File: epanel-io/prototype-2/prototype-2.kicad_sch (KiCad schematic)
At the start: 30 parts, among them J1 Conn_01x05_Male, J2 Screw_Terminal_01x04, J3 Screw_Terminal_01x04, J4 Screw_Terminal_01x02, Q1 IRF830, Q2 IRF830, SW1 SW_Push, U1 Pico, U2 4N35, U3 4N35, U4 H11AA1, U5 H11AA1, U6 H11AA1

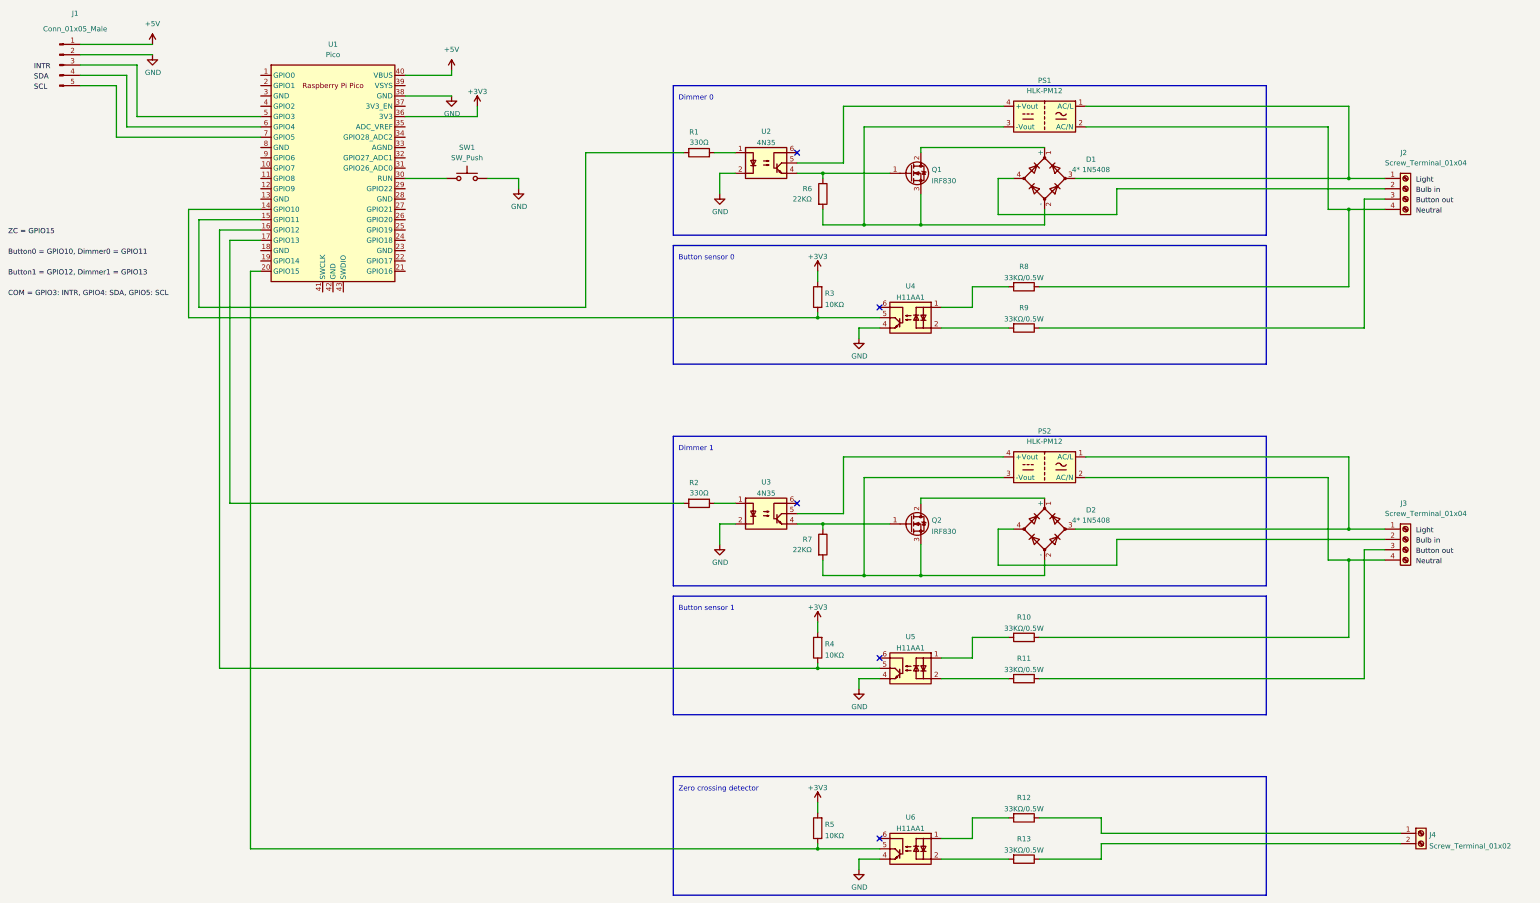
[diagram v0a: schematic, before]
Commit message: remove pico from pcb
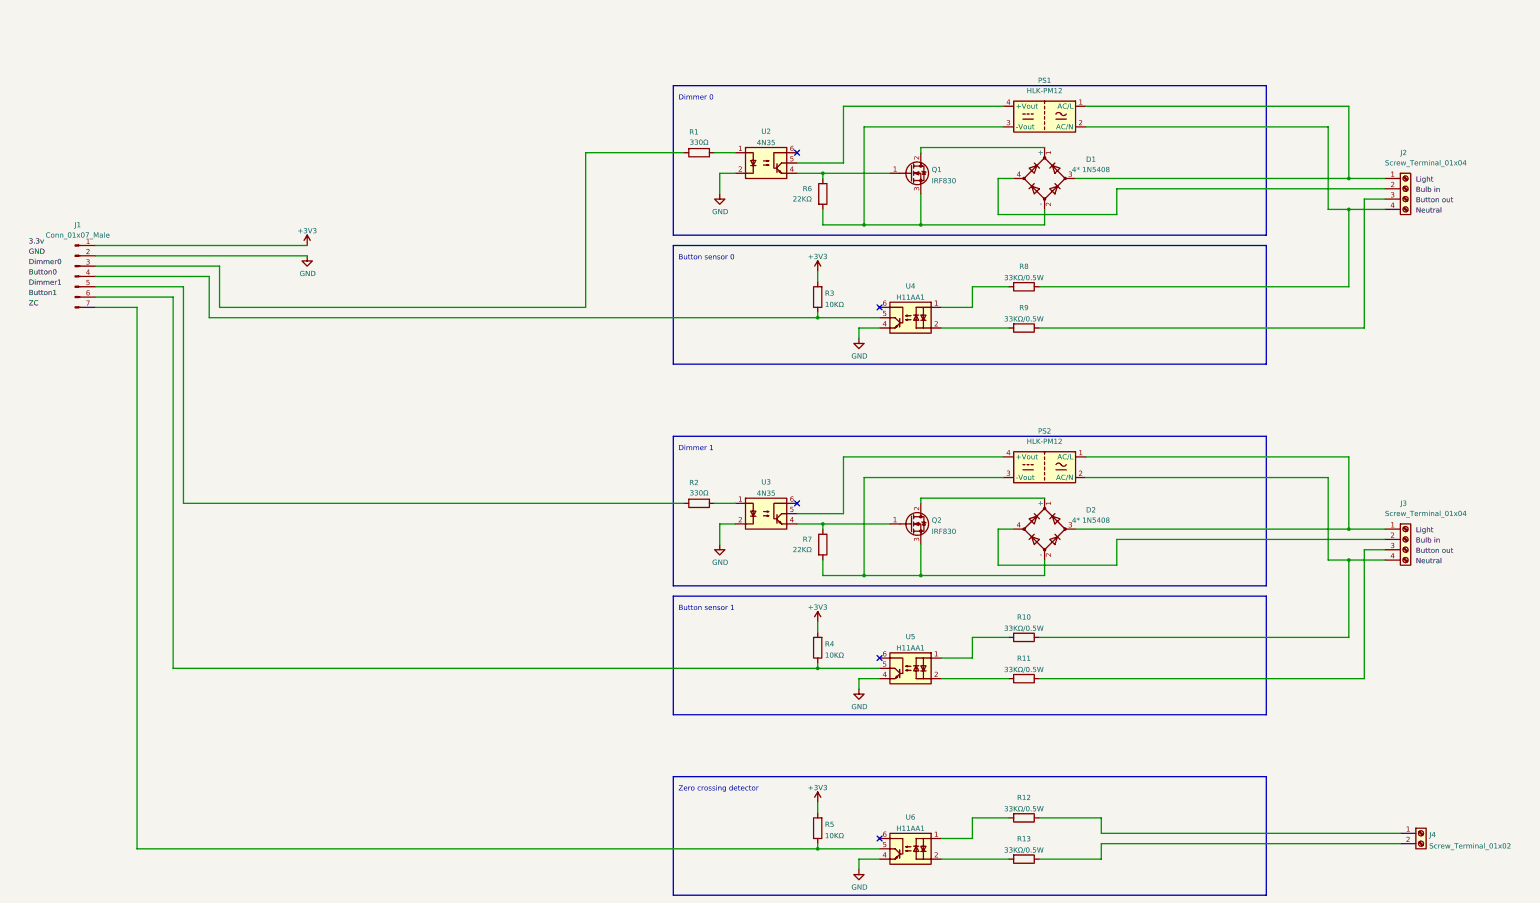
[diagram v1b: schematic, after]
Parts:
- removed J1: Conn_01x05_Male, Connector_PinHeader_2.54mm:PinHeader_1x05_P2.54mm_Vertical, symbol Connector:Conn_01x05_Male
- removed SW1: SW_Push, Button_Switch_SMD:SW_SPST_REED_CT05-XXXX-J1, symbol Switch:SW_Push
- removed U1: Pico, MCU_RaspberryPi_and_Boards:RPi_Pico_SMD_TH, symbol MCU_RaspberryPi_and_Boards:Pico
- added J1: Conn_01x07_Male, symbol Connector:Conn_01x07_Male
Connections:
- net +3V3: now also J1.1 (Pin_1)
- net GND: now also J1.2 (Pin_2)
- net at R4.1, U5.5: now also J1.6 (Pin_6)
- net at R1.2: now also J1.3 (Pin_3)
- net at R3.1, U4.5: now also J1.4 (Pin_4)
- net at R2.2: now also J1.5 (Pin_5)
- net at R5.1, U6.5: now also J1.7 (Pin_7)
